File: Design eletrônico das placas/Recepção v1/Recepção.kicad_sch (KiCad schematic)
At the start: 19 parts, among them J1 Valvula, Q1 AO3401A, Q2 AO3400A, U1 TPS63020DSJR, U2 DEVKIT_V1_ESP32-WROOM-32, U3 PC817

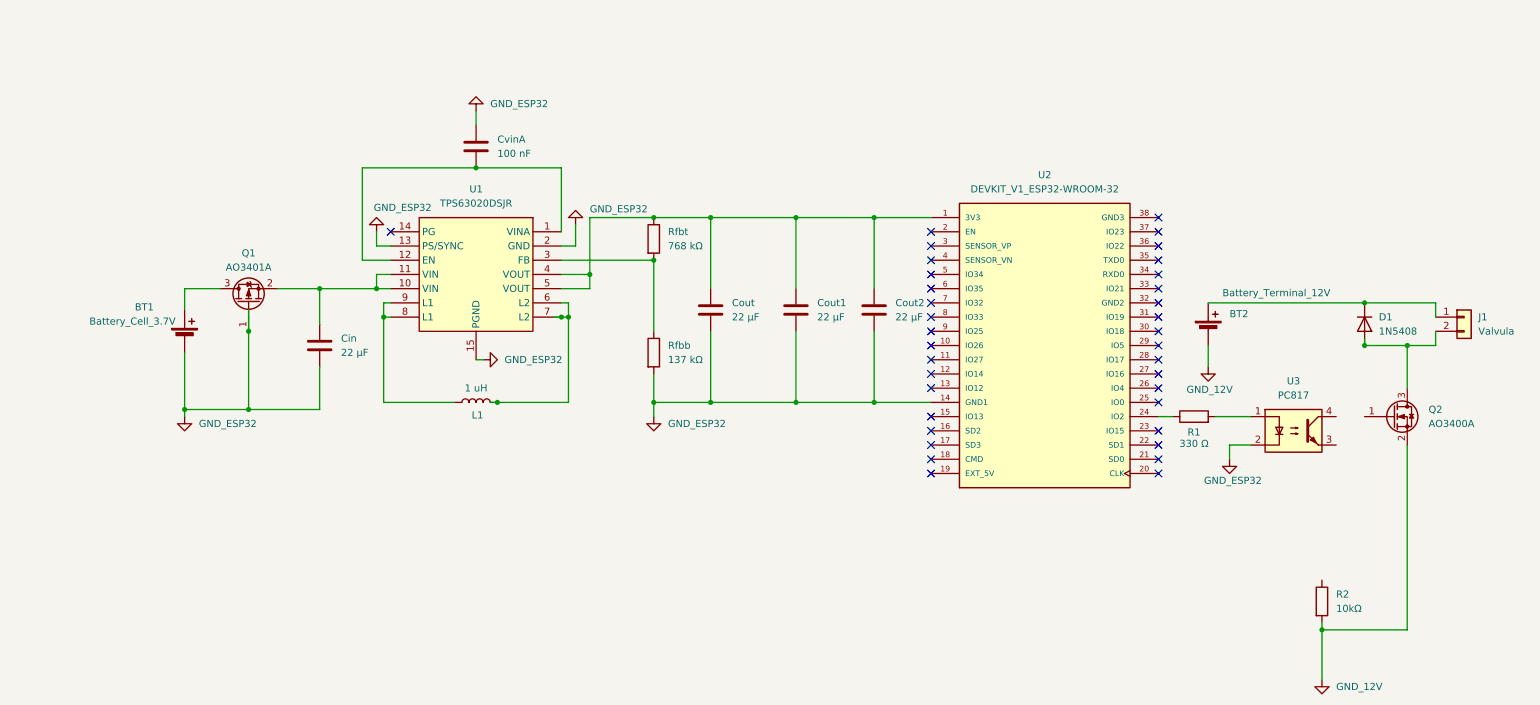
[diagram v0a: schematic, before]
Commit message: Topologia com optoacoplador completa
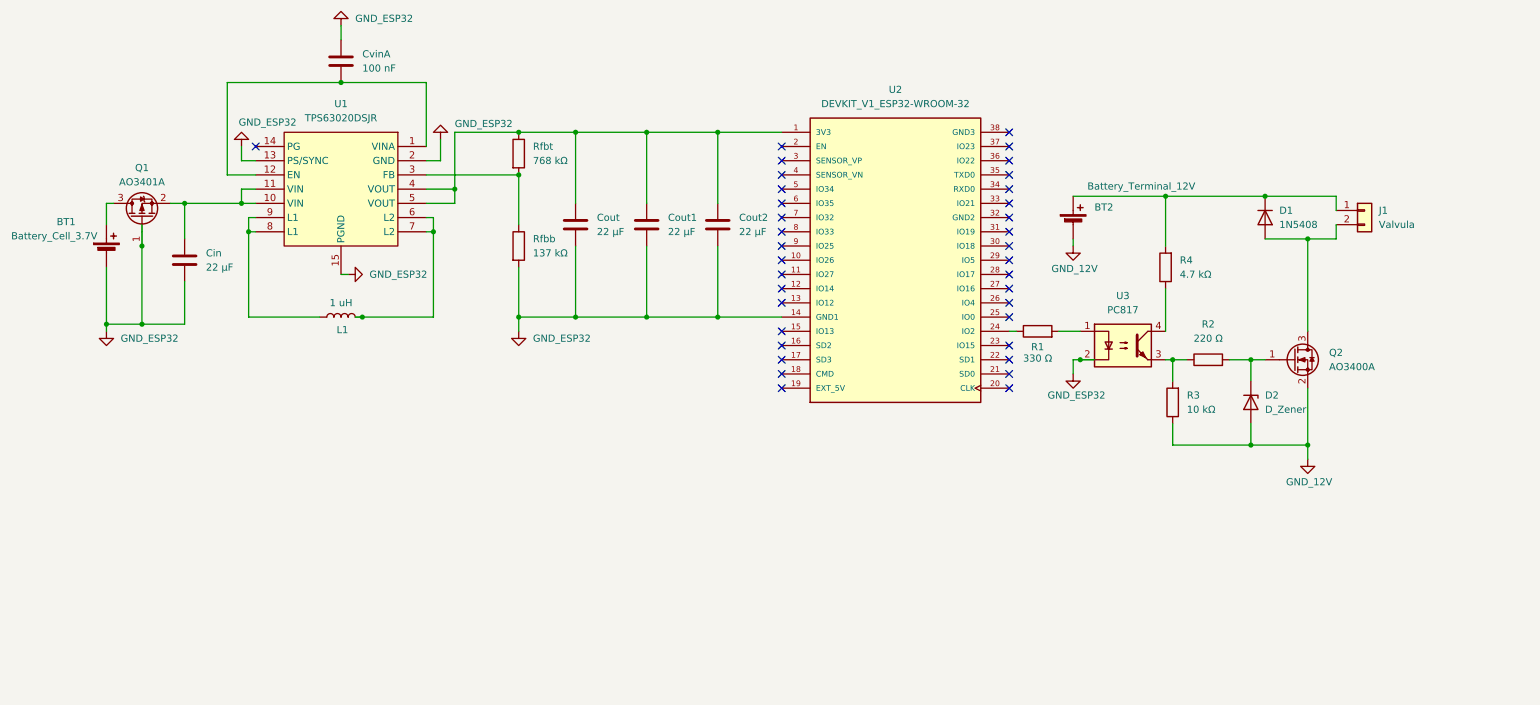
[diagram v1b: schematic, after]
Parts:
- added D2: D_Zener, Diode_THT:D_DO-35_SOD27_P7.62mm_Horizontal, symbol Device:D_Zener
- added R3: 10 kΩ, Package_DIP:DIP-8_W7.62mm, symbol Device:R
- added R4: 4.7 kΩ, Package_DIP:DIP-8_W7.62mm, symbol Device:R
- R2: value 10kΩ -> 220 Ω; footprint Resistor_THT:R_Axial_DIN0207_L6.3mm_D2.5mm_P7.62mm_Horizontal -> Package_DIP:DIP-8_W7.62mm
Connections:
- net GND_12V: now also D2.2 (A), R3.1; no longer R2.2
- net at BT2.1 (+), D1.1 (K), J1.1 (Pin_1): now also R4.2
- net at R2.1: now also U3.3, R3.2
- net at U3.4: now also R4.1
- net at Q2.1 (G): now also R2.2, D2.1 (K)
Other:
- moved on the sheet: BT1, BT2, Cin, Cout, Cout1, Cout2, CvinA, D1, J1, L1, Q1, Q2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
